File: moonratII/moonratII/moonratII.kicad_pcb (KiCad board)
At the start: 2 copper layers, 100 x 65 mm, 37 parts, among them J1 Barrel_Jack_Switch_SMT, J10 Conn_02x05_Odd_Even, J11 Screw_Terminal_01x02, J2 SSD1306 OLED, J3 PinHeader_1x06_P2.54mm_Vertic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, J4 PinHeader_1x08_P2.54mm_Vertic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, J5 Conn_02x05_Odd_Even, J6 Screw_Terminal_01x06, J7 PinHeader_1x08_P2.54mm_Vertic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, J8 PinHeader_1x10_P2.54mm_Vertic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, J9 Screw_Terminal_01x06, Q1 IRF520N, Q2 BSS138, SW1 6mm 2 Pin Tact NO Breadboard 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, SW2 6mm 2 Pin Tact NO Breadboard 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, SW3 6mm 2 Pin Tact NO Breadboard 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, U1 TMP36xS

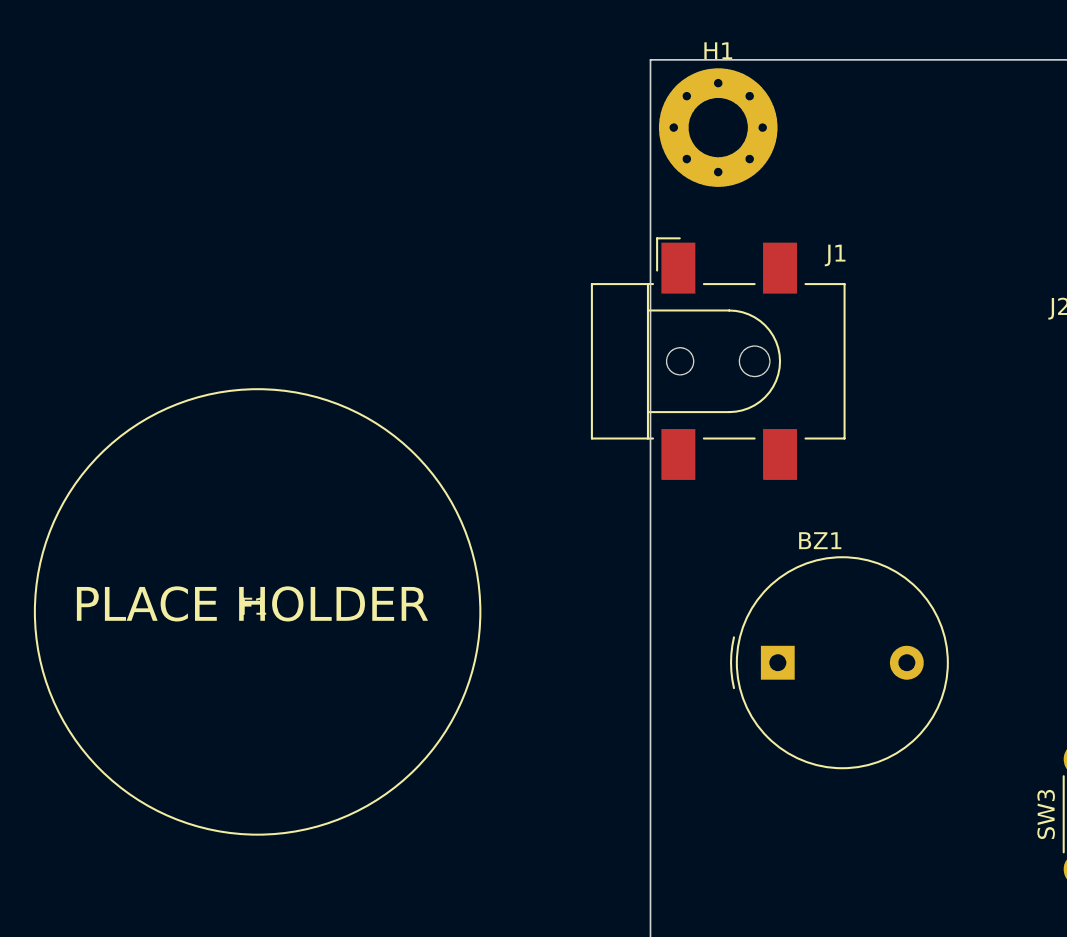
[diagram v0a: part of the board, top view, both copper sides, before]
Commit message: Created a footprint fuse BSMD1812
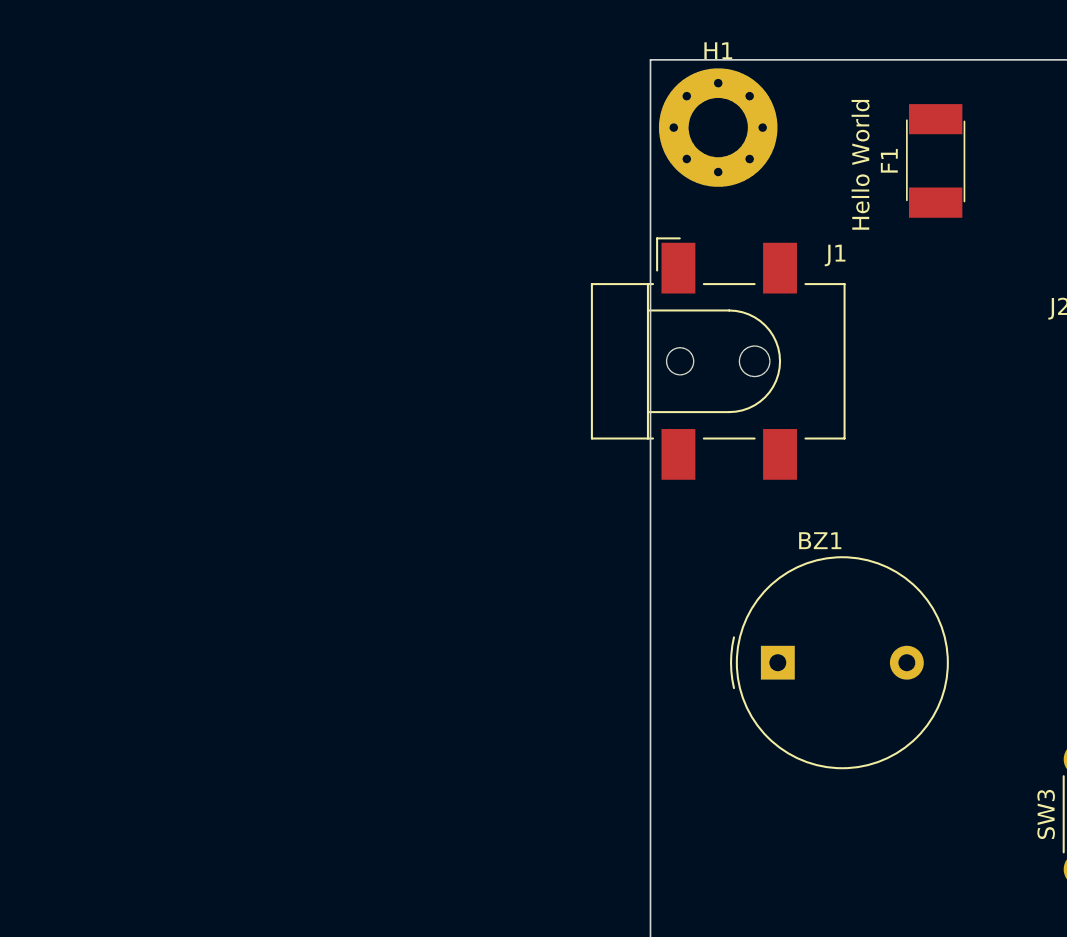
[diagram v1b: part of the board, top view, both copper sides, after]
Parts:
- F1: footprint GeneralPurposeAlarmDevicePCB:PlaceHolderOpossum -> GeneralPurposeAlarmDevicePCB:Fuse_BSMD_1812
- moved F1 48.4 mm to (116.8, 66.0), turned to 90 degrees
